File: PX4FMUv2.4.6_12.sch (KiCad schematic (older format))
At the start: 33 parts, among them M3_MOUNT1101 MOUNT-HOLE3.1MM, M3_MOUNT1102 MOUNT-HOLE3.1MM, M3_MOUNT1103 MOUNT-HOLE3.1MM, M3_MOUNT1104 MOUNT-HOLE3.1MM

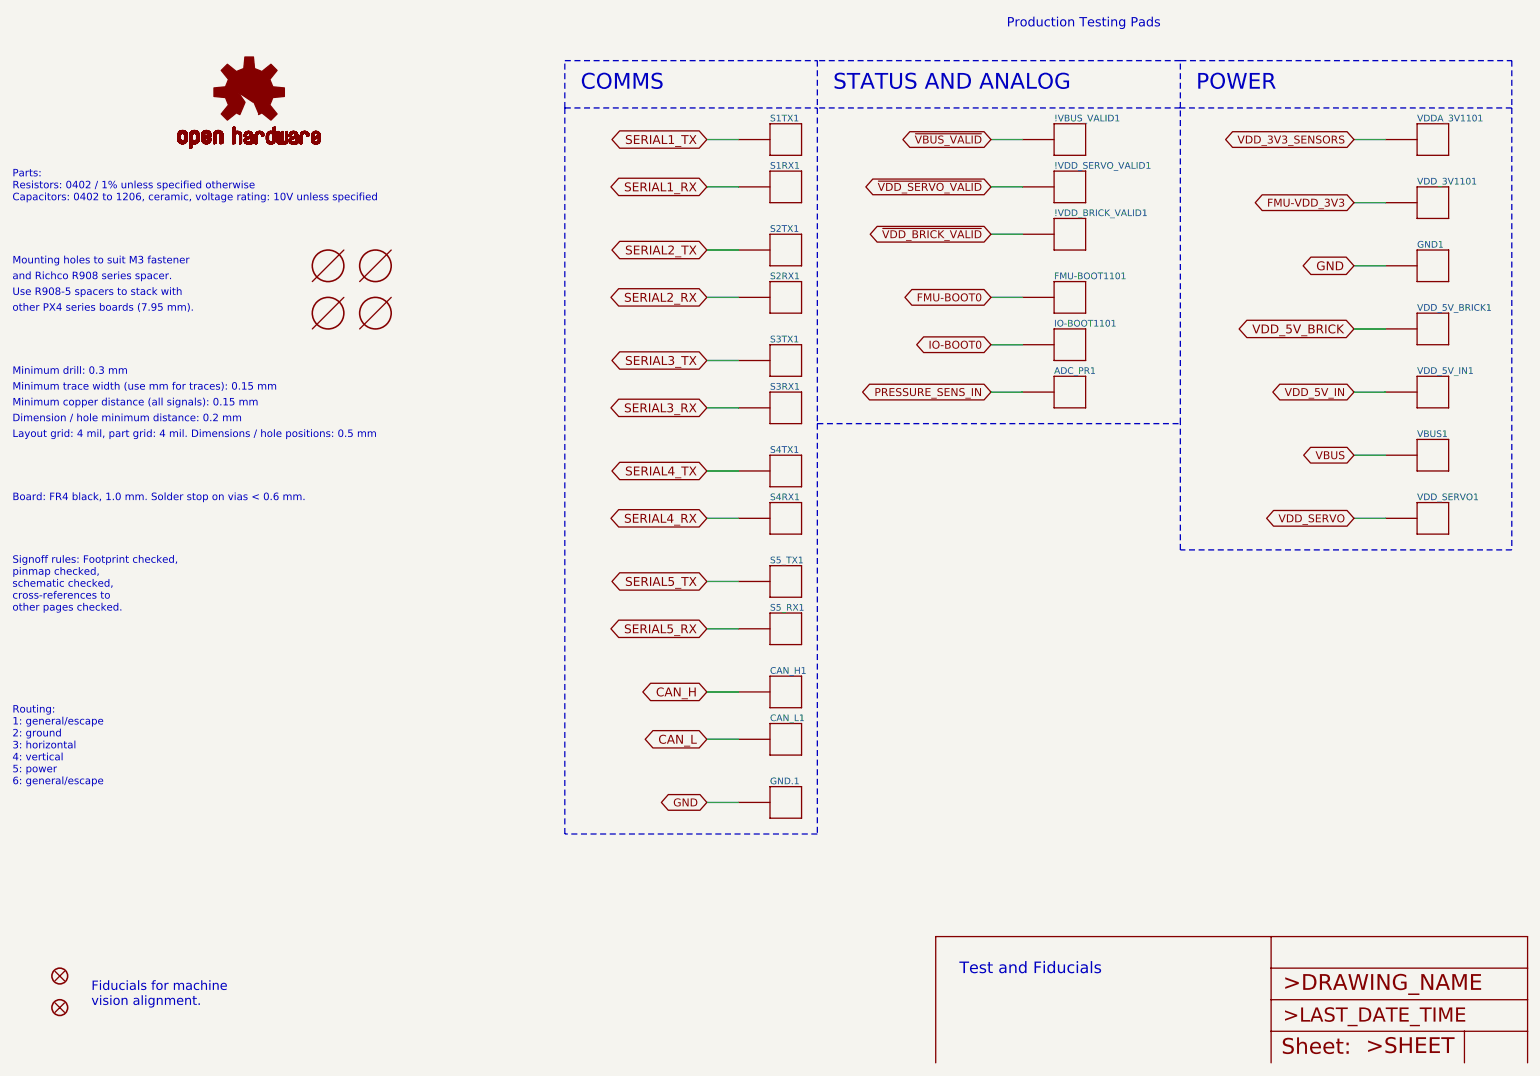
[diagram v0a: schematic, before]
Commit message: removed some things
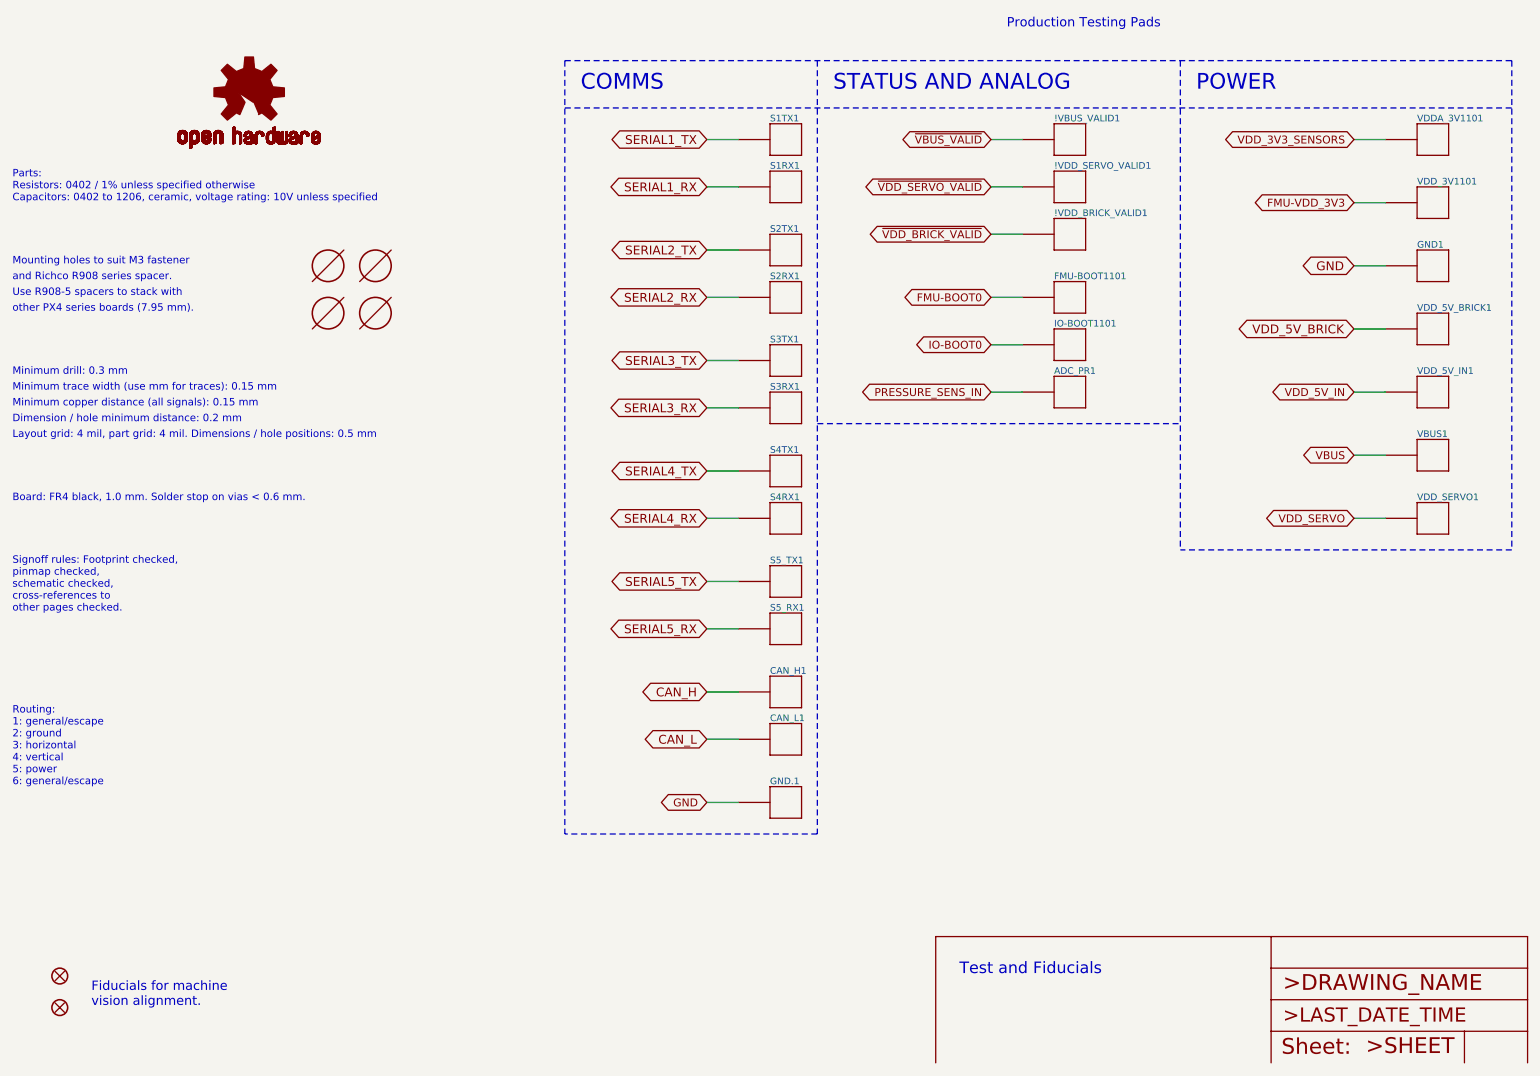
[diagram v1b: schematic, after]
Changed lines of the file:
@@
 EESchema Schematic File Version 4
+LIBS:PX4FMUv2.4.6-cache
 EELAYER 26 0
 EELAYER END
 $Descr User 11818 8333
 encoding utf-8
-Sheet 1 13
+Sheet 13 13
 Title ""
 Date ""
@@
 Parts:\nResistors: 0402 / 1% unless specified otherwise\nCapacitors: 0402 to 1206, ceramic, voltage rating: 10V unless specified
 Wire Notes Line
-	4900 1300 6500 1300
-Wire Notes Line
-	10900 1300 10900 4100
-Wire Notes Line
 	10900 4100 8800 4100
 Wire Notes Line
-	8800 4100 8800 3300
-Wire Notes Line
-	8800 3300 8800 1300
-Wire Notes Line
-	8800 1300 6500 1300
-Wire Notes Line
-	6500 1300 6500 3300
-Wire Notes Line
-	6500 3300 6500 5900
-Wire Notes Line
 	6500 5900 4900 5900
 Wire Notes Line
-	4900 5900 4900 1300
-Wire Notes Line
 	6500 3300 8800 3300
-Wire Notes Line
-	4900 1300 4900 1000
-Wire Notes Line
-	4900 1000 6500 1000
-Wire Notes Line
-	8800 1000 10900 1000
-Wire Notes Line
-	10900 1000 10900 1300
-Wire Notes Line
-	10900 1300 8800 1300
-Wire Notes Line
-	8800 1300 8800 1000
-Wire Notes Line
-	8800 1000 6500 1000
-Wire Notes Line
-	6500 1000 6500 1300
 Text Notes 5000 1200 0    100  ~ 0
 COMMS
@@
 Text Notes 6600 1200 0    100  ~ 0
 STATUS AND ANALOG
+Wire Notes Line
+	10900 1000 10900 4100
+Wire Notes Line
+	4900 1000 4900 5900
+Wire Notes Line
+	4900 1000 10900 1000
+Wire Notes Line
+	4900 1300 10900 1300
+Wire Notes Line
+	8800 1000 8800 4100
+Wire Notes Line
+	6500 1000 6500 5900
 $EndSCHEMATC
